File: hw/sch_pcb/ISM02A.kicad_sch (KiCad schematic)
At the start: 55 parts, among them J1 JUMP_3X2, J10 HEADER_2x01_PARALLEL, J11 HEADER_2x01_PARALLEL, J12 SMA, J13 HEADER_2x01_PARALLEL, J15 HEADER_2x01_PARALLEL, J2 HEADER_2x01_PARALLEL, J3 HEADER_2x01_PARALLEL, J4 HEADER_2x01_PARALLEL, J5 HEADER_2x01_PARALLEL, J6 HEADER_2x01_PARALLEL, J7 HEADER_2x01_PARALLEL, J8 HEADER_2x01_PARALLEL, J9 HEADER_2x01_PARALLEL, M1 HOLE, M2 HOLE, M3 HOLE, M4 HOLE, U1 SX1262, U2 MIC5504-3.3YM5, Y1 32MHz

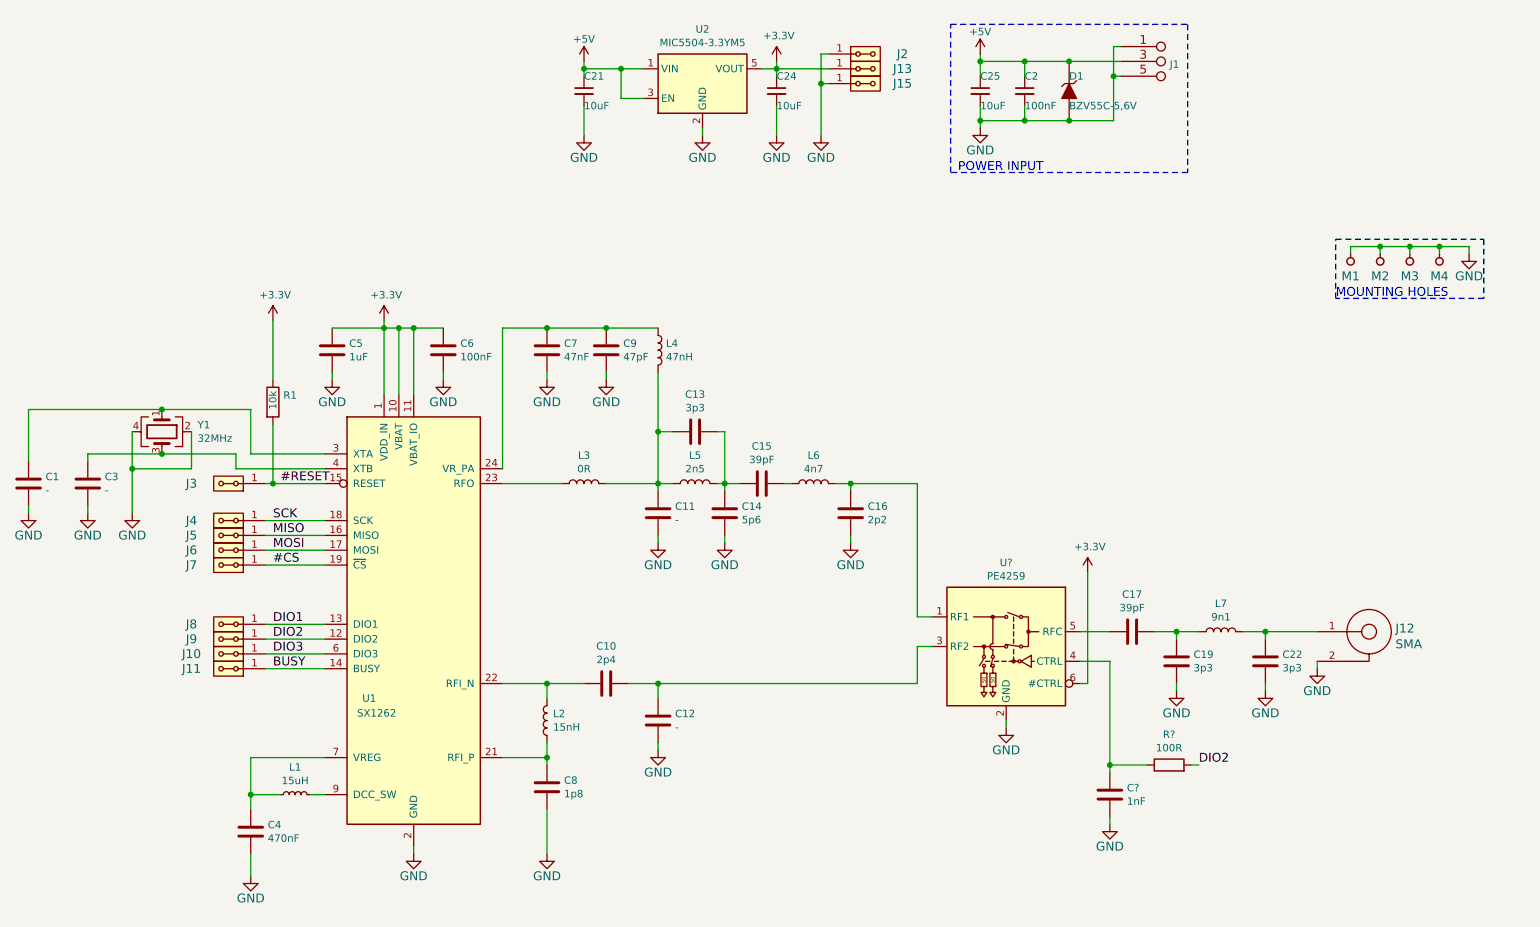
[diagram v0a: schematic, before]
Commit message: Revert "Edit"
This reverts commit 3bfea5ab87054fd9b05002ed626080fed2685c40.
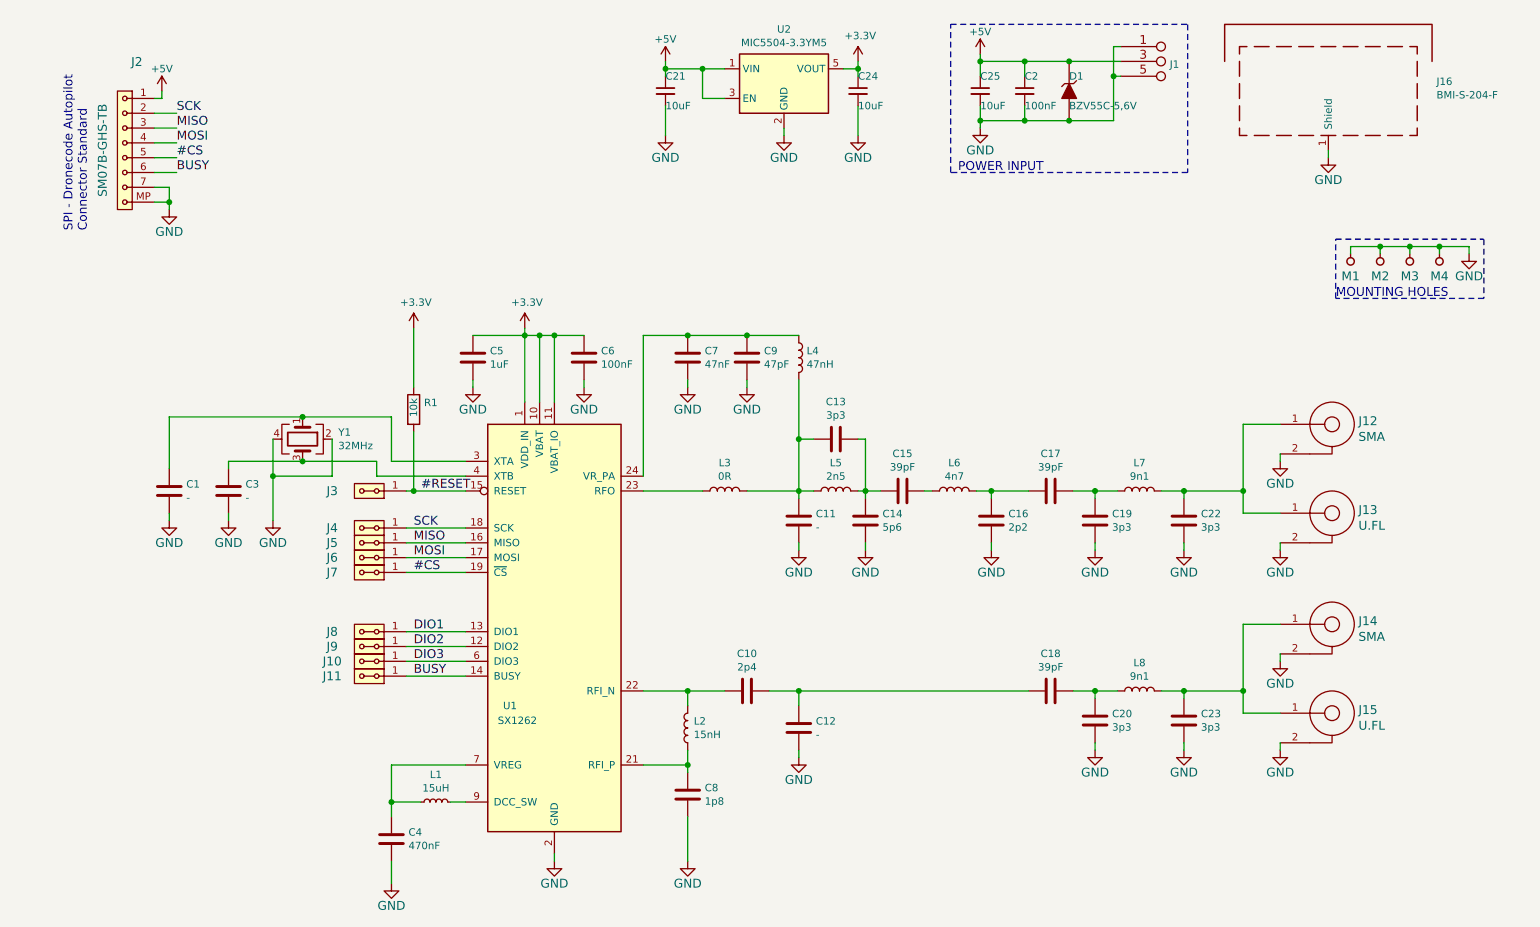
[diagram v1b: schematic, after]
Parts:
- removed C?: 1nF, symbol Device:C
- removed J13, J15, J2: HEADER_2x01_PARALLEL, Mlab_Pin_Headers:Straight_2x01, symbol ISM02A-rescue:HEADER_2x01_PARALLEL-MLAB_HEADER
- removed R?: 100R, symbol Device:R
- removed U?: PE4259, Package_TO_SOT_SMD:SOT-363_SC-70-6, symbol MLAB_IO:PE4259
- added C18: 39pF, Capacitor_SMD:C_0603_1608Metric_Pad1.05x0.95mm_HandSolder, symbol ISM02A-rescue:C-Device-ISM02A-rescue
- added C20, C23: 3p3, Capacitor_SMD:C_0603_1608Metric_Pad1.05x0.95mm_HandSolder, symbol ISM02A-rescue:C-Device-ISM02A-rescue
- added J13, J15: U.FL, Connector_Coaxial:U.FL_Hirose_U.FL-R-SMT-1_Vertical, symbol ISM02A-rescue:SMA-MLAB_CONNECTORS
- added J14: SMA, Mlab_CON:SMA6251A13G50, symbol ISM02A-rescue:SMA-MLAB_CONNECTORS
- added J16: BMI-S-204-F, MYLIB:BMI-S-204-F, symbol ISM02A-rescue:RF_Shield_Two_Pieces-device
- added J2: SM07B-GHS-TB, Connector_JST:JST_GH_SM07B-GHS-TB_1x07-1MP_P1.25mm_Horizontal, symbol ISM02A-rescue:SM07B-GHS-TB-MLAB_CONNECTORS_JST-ISM02A-rescue
- added L8: 9n1, Inductor_SMD:L_0402_1005Metric, symbol ISM02A-rescue:L-Device-ISM02A-rescue
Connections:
- net #CS: now also J2.5
- net +5V: now also J2.1
- net BUSY: now also J2.6
- net GND: now also C20.1, C23.1, J13.2, J14.2, J15.2, J16.1 (Shield), J2.7, J2.MP
- net MISO: now also J2.3
- net MOSI: now also J2.4
- net SCK: now also J2.2
- net at C22.2, J12.1, L7.2: now also J13.1
- net at C16.1, L6.2: now also C17.2
- net at C10.1, C12.1: now also C18.2
- new net: C23.2, J14.1, J15.1, L8.2
- new net: C18.1, C20.2, L8.1
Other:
- note added: "SPI - Dronecode Autopilot Connector Standard"
- moved on the sheet: C1, C10, C11, C12, C13, C14, C15, C16, C17, C19, C21, C22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
